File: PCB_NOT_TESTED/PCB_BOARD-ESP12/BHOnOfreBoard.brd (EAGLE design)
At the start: 53 x 55 mm, 23 parts, among them J1 4p, J6 8p, J7 8p, K1 OMRON-G3MB-202P-SSR2, K2 OMRON-G3MB-202P-SSR2, Q1 S8050, Q2 S8050, U1 LM1117, U2 esp12

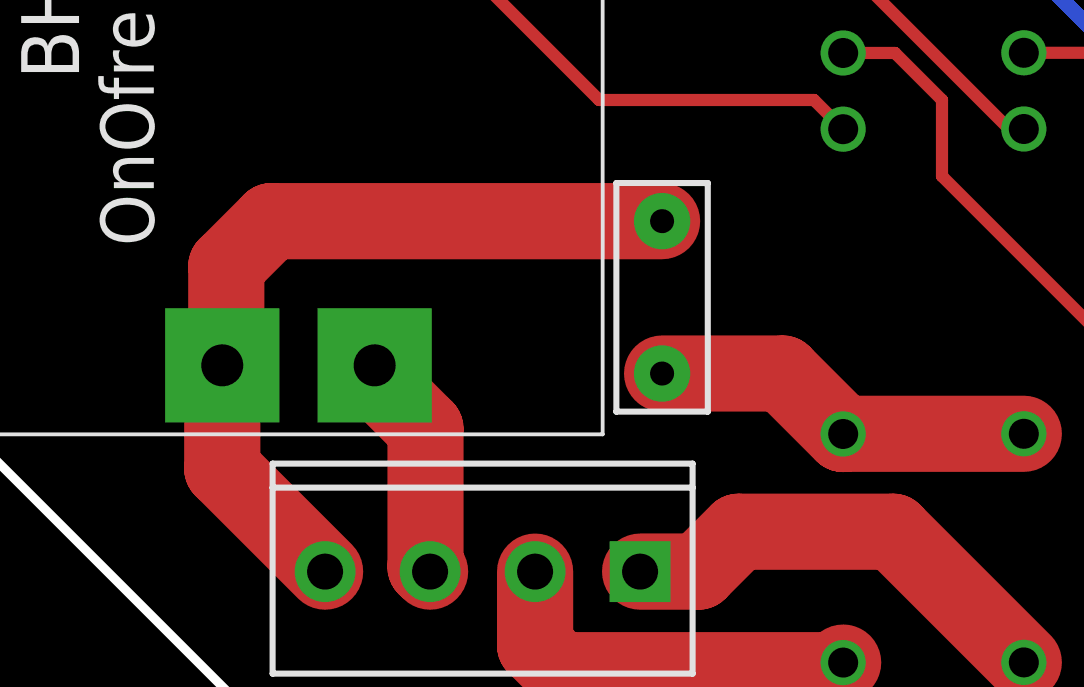
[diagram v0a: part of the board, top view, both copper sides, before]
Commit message: OnOfre Square rev2 80% pronto
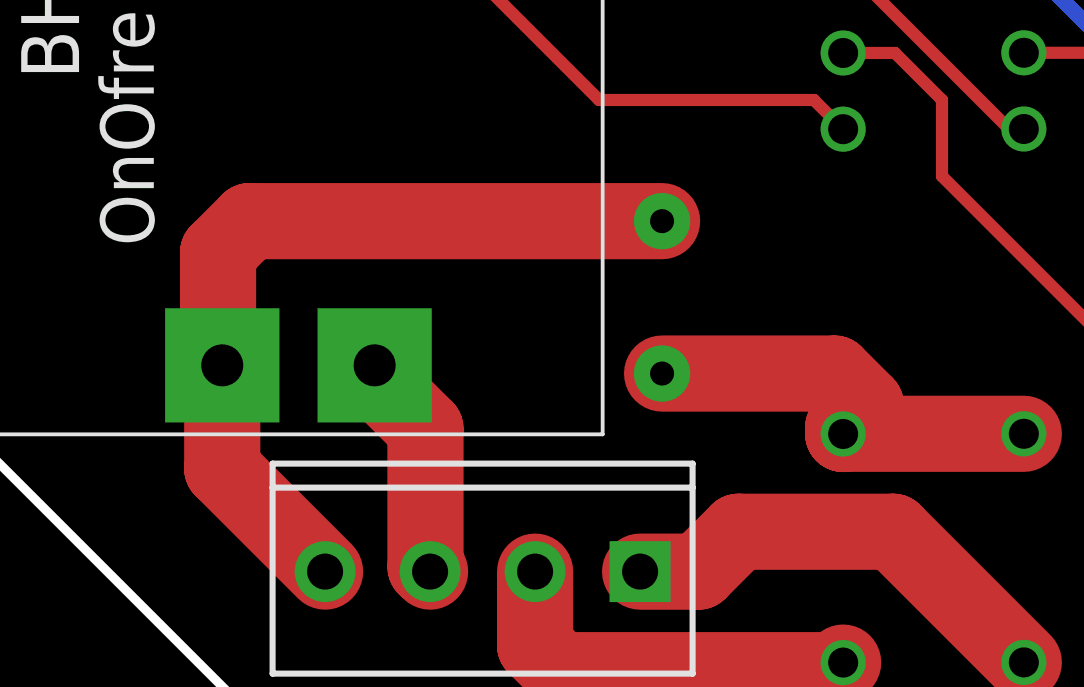
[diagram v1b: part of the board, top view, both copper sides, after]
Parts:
- flipped F1 to the bottom
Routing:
- net NEUTRAL_IN_FUSED: track 12.9 -> 14.5 mm
- net NEUTRAL_IN: track 26.8 -> 27.3 mm
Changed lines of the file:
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@@
 <attribute name="OC_NEWARK" value="14N9588" x="30.9955875" y="15.53723125" size="1.778" layer="28" rot="MR90" display="off"/>
 </element>
-<element name="F1" library="SparkFun-Fuses" library_urn="urn:adsk.eagle:library:517" package="PTH" package3d_urn="urn:adsk.eagle:package:38574/1" value="FUSE 2A" x="24.959440625" y="15.011509375" smashed="yes" rot="R270">
-<attribute name="PROD_ID" value="RES-08490" x="24.959440625" y="15.011509375" size="1.778" layer="27" rot="R270" display="off"/>
-<attribute name="VALUE" x="27.416103125" y="16.2050875" size="0.6096" layer="27" font="vector" ratio="20" rot="R270" align="top-center"/>
+<element name="F1" library="SparkFun-Fuses" library_urn="urn:adsk.eagle:library:517" package="PTH" package3d_urn="urn:adsk.eagle:package:38574/1" value="FUSE 2A" x="24.959440625" y="15.011509375" smashed="yes" rot="MR270">
+<attribute name="PROD_ID" value="RES-08490" x="24.959440625" y="15.011509375" size="1.778" layer="28" rot="MR270" display="off"/>
+<attribute name="VALUE" x="22.502778125" y="16.2050875" size="0.6096" layer="28" font="vector" ratio="20" rot="MR270" align="top-center"/>
 </element>
 <element name="Q1" library="semicon-smd-ipc" library_urn="urn:adsk.eagle:library:353" package="SOT23" package3d_urn="urn:adsk.eagle:package:26310/1" value="S8050 " x="45.795765625" y="12.608365625" smashed="yes">
@@
 <contactref element="J1" pad="4"/>
 <contactref element="U$2" pad="AC1"/>
-<wire x1="10.29839375" y1="9.297371875" x2="10.29839375" y2="12.744771875" width="2.54" layer="1"/>
+<wire x1="10.29839375" y1="12.744771875" x2="10.29839375" y2="9.297371875" width="2.54" layer="1"/>
 <wire x1="10.29839375" y1="9.297371875" x2="13.7265875" y2="5.869178125" width="2.54" layer="1"/>
-<wire x1="24.959440625" y1="17.551509375" x2="11.931965625" y2="17.551509375" width="2.54" layer="1"/>
-<wire x1="11.931965625" y1="17.551509375" x2="10.433234375" y2="16.052778125" width="2.54" layer="1"/>
-<wire x1="10.433234375" y1="12.8796125" x2="10.433234375" y2="16.052778125" width="2.54" layer="1"/>
-<wire x1="10.29839375" y1="12.744771875" x2="10.433234375" y2="12.8796125" width="2.54" layer="1"/>
+<wire x1="24.959440625" y1="17.551509375" x2="11.201509375" y2="17.551509375" width="2.54" layer="1"/>
+<wire x1="11.201509375" y1="17.551509375" x2="10.16" y2="16.51" width="2.54" layer="1"/>
+<wire x1="10.16" y1="16.51" x2="10.16" y2="12.883165625" width="2.54" layer="1"/>
+<wire x1="10.16" y1="12.883165625" x2="10.29839375" y2="12.744771875" width="2.54" layer="1"/>
 </signal>
 <signal name="FASE">
@@
 <contactref element="K2" pad="2"/>
 <contactref element="K1" pad="2"/>
-<wire x1="24.959440625" y1="12.471509375" x2="28.981309375" y2="12.471509375" width="2.54" layer="1"/>
-<wire x1="30.9955875" y1="10.45723125" x2="28.981309375" y2="12.471509375" width="2.54" layer="1"/>
 <wire x1="37.017684375" y1="10.463271875" x2="31.001628125" y2="10.463271875" width="2.54" layer="1"/>
 <wire x1="31.001628125" y1="10.463271875" x2="30.9955875" y2="10.45723125" width="2.54" layer="1"/>
+<wire x1="24.959440625" y1="12.471509375" x2="30.708490625" y2="12.471509375" width="2.54" layer="1"/>
+<wire x1="31.75" y1="11.43" x2="30.708490625" y2="12.471509375" width="2.54" layer="1"/>
+<wire x1="30.9955875" y1="10.45723125" x2="30.9955875" y2="10.6755875" width="2.54" layer="1"/>
+<wire x1="30.9955875" y1="10.6755875" x2="31.75" y2="11.43" width="2.54" layer="1"/>
 </signal>
 <signal name="N$2">
